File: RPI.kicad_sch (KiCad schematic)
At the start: 30 parts, among them J1 Conn_01x02_Male, J2 GPIO, J5 Conn_01x06, J6 Conn_01x04, J7 Conn_01x03, J8 Conn_01x02, J9 Conn_01x02, Q1 IRF9540N, Q2 IRF9540N, Q3 BC856BDW1, Q4 DMMT5401-7-F, SW1 SW_SPDT, SW2 SW_SPDT, U1 LM1085-ADJ, U2 LM1085-ADJ

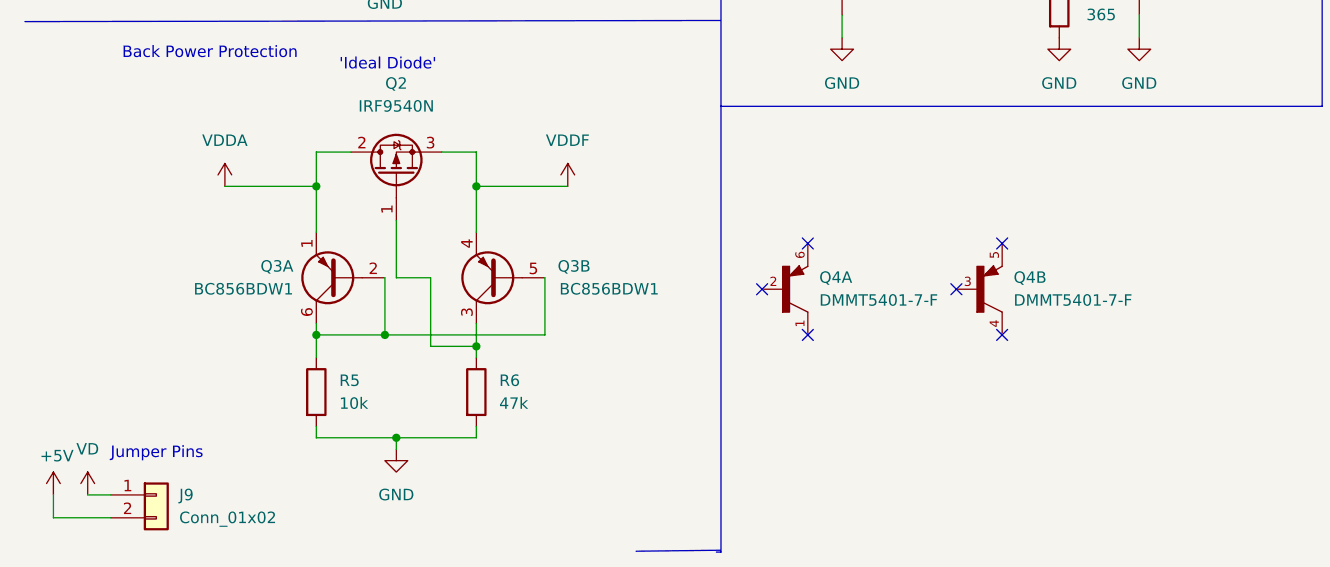
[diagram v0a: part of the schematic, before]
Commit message: V2 Ready for checking
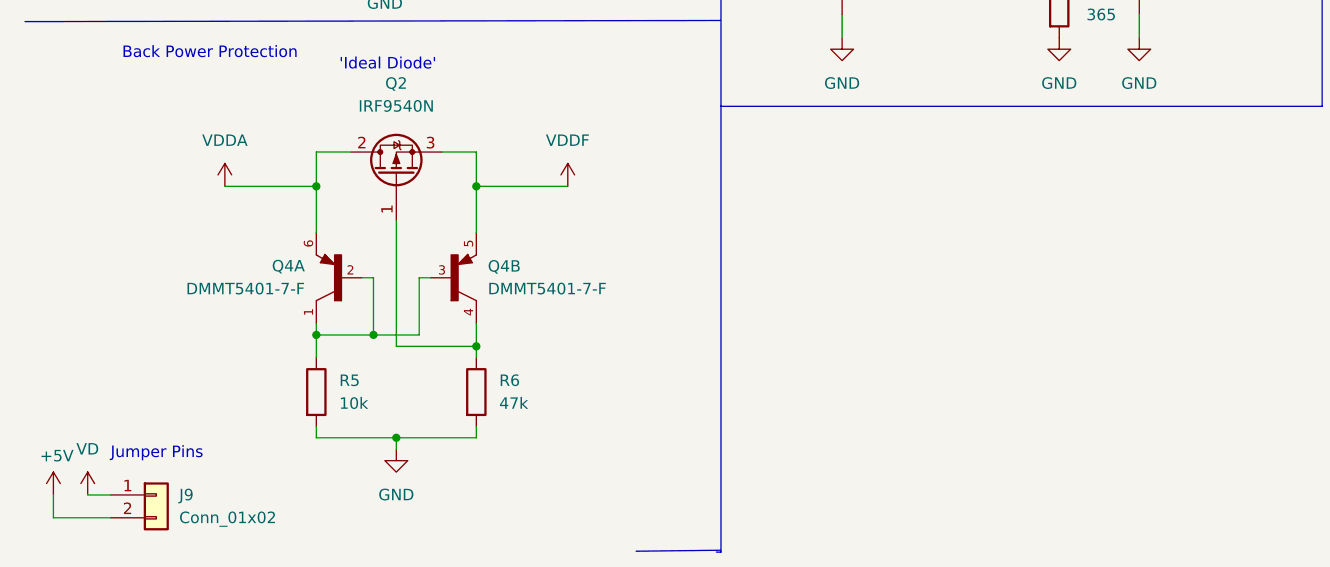
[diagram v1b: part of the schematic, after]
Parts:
- removed Q3: BC856BDW1, Package_TO_SOT_SMD:SOT-363_SC-70-6, symbol Transistor_BJT:BC856BDW1
- U1, U2: footprint RPi_Hat:LM1085-5.0 -> Package_TO_SOT_THT:TO-220-3_Vertical
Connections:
- net VD: now also Q4.5
- net VDDA: now also Q4.6
- net at Q4.3: now also Q4.1, Q4.2, R5.1
- net at Q4.4: now also Q2.1 (G), R6.1
- no-connect marks 9 -> 3
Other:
- moved on the sheet: Q4A, Q4B
